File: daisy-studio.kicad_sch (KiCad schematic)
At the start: 0 parts

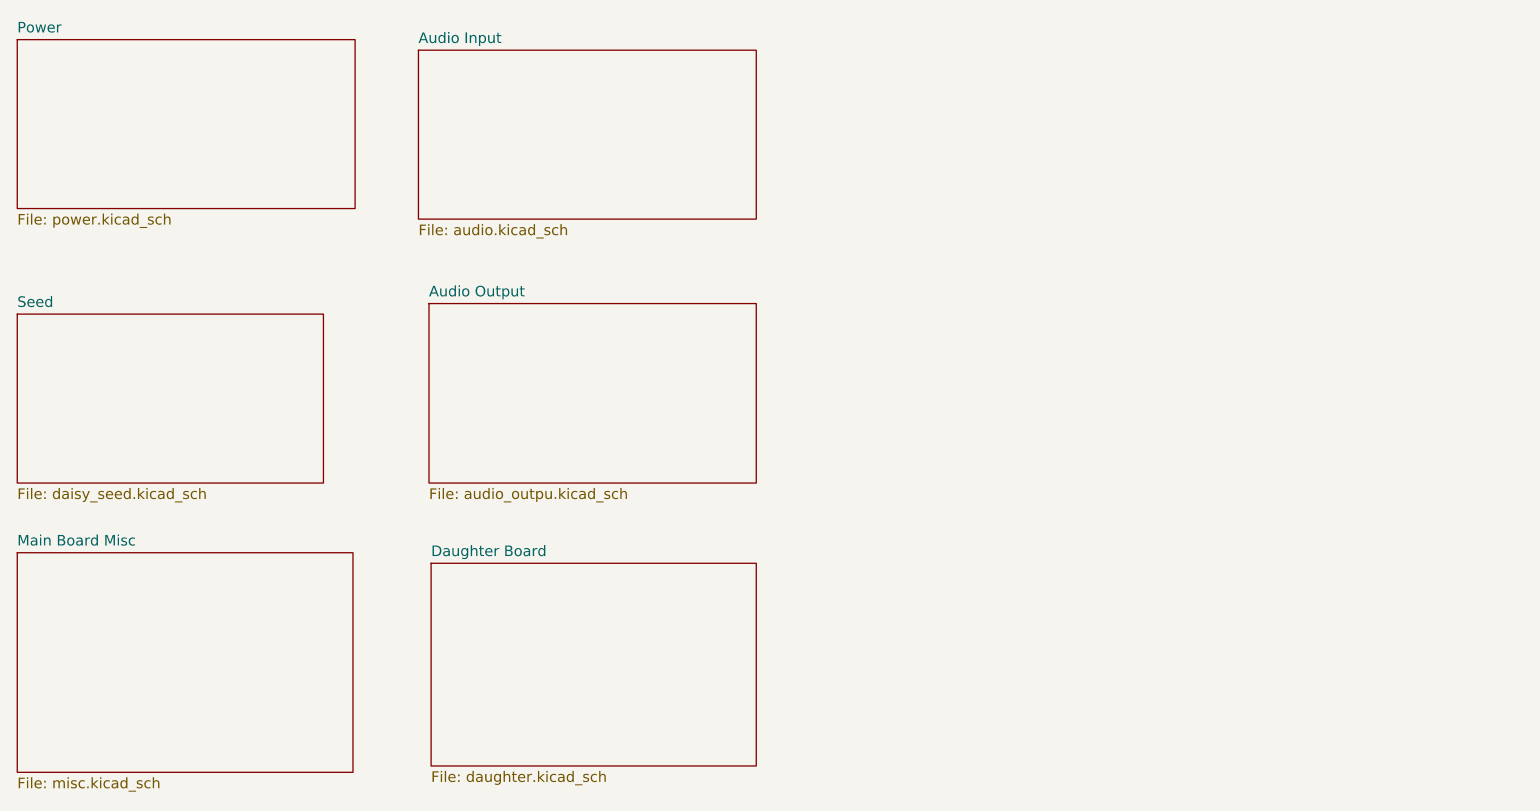
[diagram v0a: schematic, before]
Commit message: WIP adding values
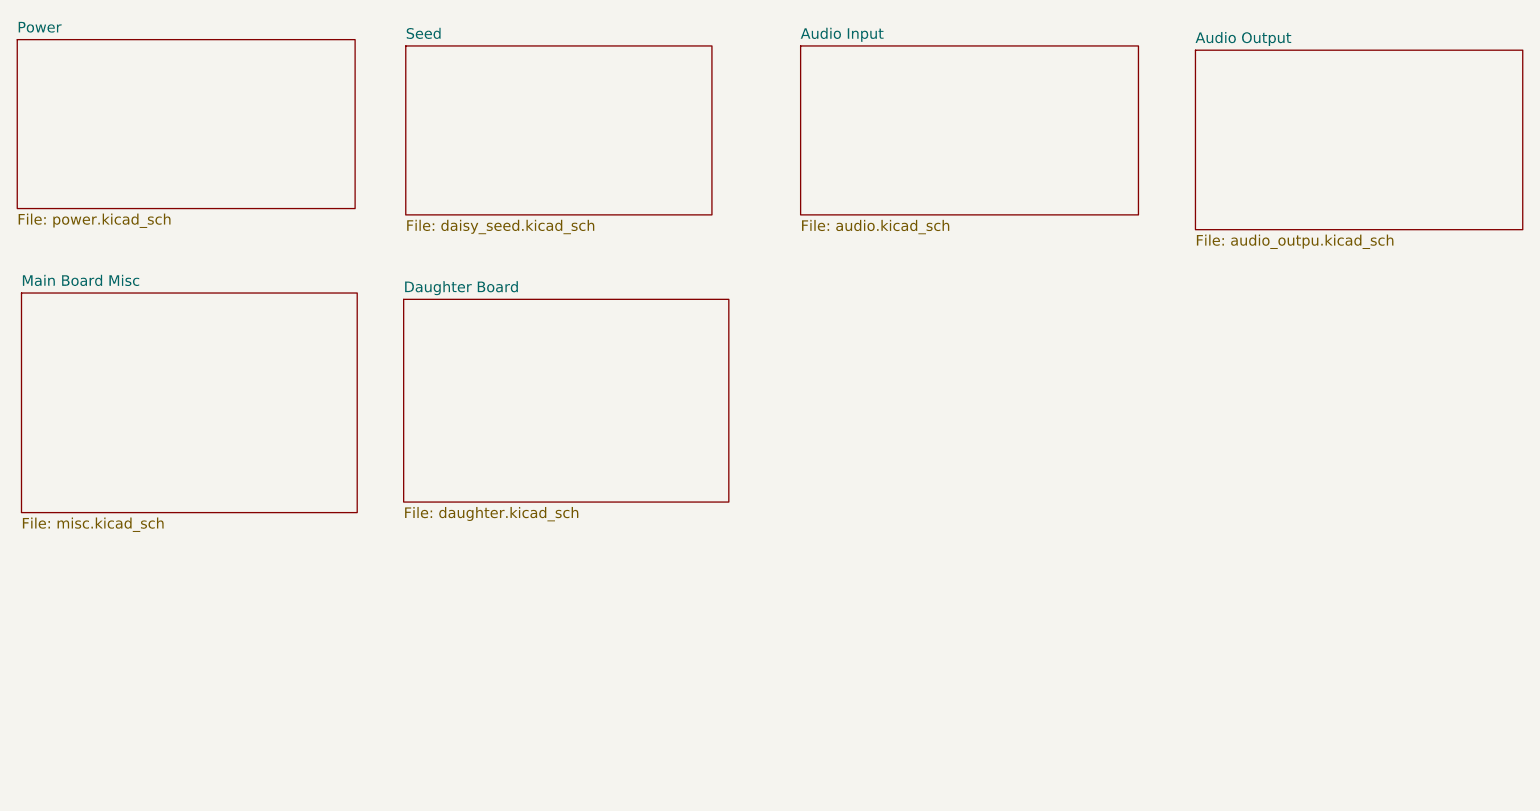
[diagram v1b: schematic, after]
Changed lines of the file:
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@@
 	)
 	(sheet
-		(at 80.01 62.23)
+		(at 172.212 31.75)
 		(size 39.37 21.59)
 		(exclude_from_sim no)
@@
 		)
 		(property "Sheetname" "Audio Output"
-			(at 80.01 61.5184 0)
+			(at 172.212 31.0384 0)
 			(effects
 				(font
@@
 		)
 		(property "Sheetfile" "audio_outpu.kicad_sch"
-			(at 80.01 84.4046 0)
+			(at 172.212 53.9246 0)
 			(effects
 				(font
@@
 	)
 	(sheet
-		(at 30.48 63.5)
+		(at 77.216 31.242)
 		(size 36.83 20.32)
 		(exclude_from_sim no)
@@
 		)
 		(property "Sheetname" "Seed"
-			(at 30.48 62.7884 0)
+			(at 77.216 30.5304 0)
 			(effects
 				(font
@@
 		)
 		(property "Sheetfile" "daisy_seed.kicad_sch"
-			(at 30.48 84.4046 0)
+			(at 77.216 52.1466 0)
 			(effects
 				(font
@@
 	)
 	(sheet
-		(at 80.264 93.472)
+		(at 76.962 61.722)
 		(size 39.116 24.384)
 		(exclude_from_sim no)
@@
 		)
 		(property "Sheetname" "Daughter Board"
-			(at 80.264 92.7604 0)
+			(at 76.962 61.0104 0)
 			(effects
 				(font
@@
 		)
 		(property "Sheetfile" "daughter.kicad_sch"
-			(at 80.264 118.4406 0)
+			(at 76.962 86.6906 0)
 			(effects
 				(font
@@
 	)
 	(sheet
-		(at 78.74 31.75)
+		(at 124.714 31.242)
 		(size 40.64 20.32)
 		(exclude_from_sim no)
@@
 		)
 		(property "Sheetname" "Audio Input"
-			(at 78.74 31.0394 0)
+			(at 124.714 30.5314 0)
 			(effects
 				(font
@@
 		)
 		(property "Sheetfile" "audio.kicad_sch"
-			(at 78.74 52.6646 0)
+			(at 124.714 52.1566 0)
 			(effects
 				(font
@@
 	)
 	(sheet
-		(at 30.48 92.202)
+		(at 30.988 60.96)
 		(size 40.386 26.416)
 		(exclude_from_sim no)
@@
 		)
 		(property "Sheetname" "Main Board Misc"
-			(at 30.48 91.4904 0)
+			(at 30.988 60.2484 0)
 			(effects
 				(font
@@
 		)
 		(property "Sheetfile" "misc.kicad_sch"
-			(at 30.48 119.2026 0)
-			(effects
-				(font
+			(at 30.988 87.9606 0)
+			(effects
+				(font
